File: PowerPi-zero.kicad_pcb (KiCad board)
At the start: 2 copper layers, 65 x 56 mm, 34 parts, among them J1 2444, J3 Conn_01x02, J6 Raspberry_Pi_2_3, J8 2444, Q1 30V 4A 44mΩ, Q2 50nA 150V 200mW 200mA, Q3 30V 4A 44mΩ, U1 XL4015

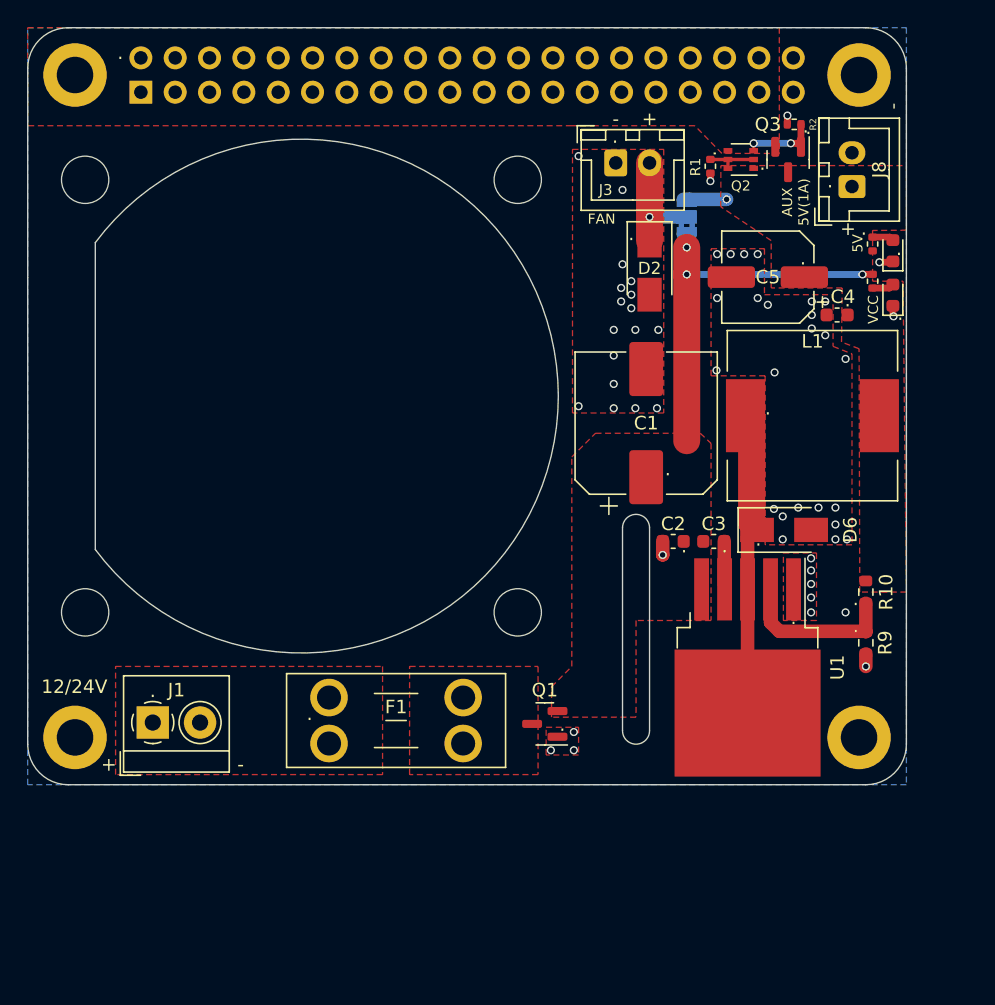
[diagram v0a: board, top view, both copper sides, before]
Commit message: Layout complete for PowerPi zero
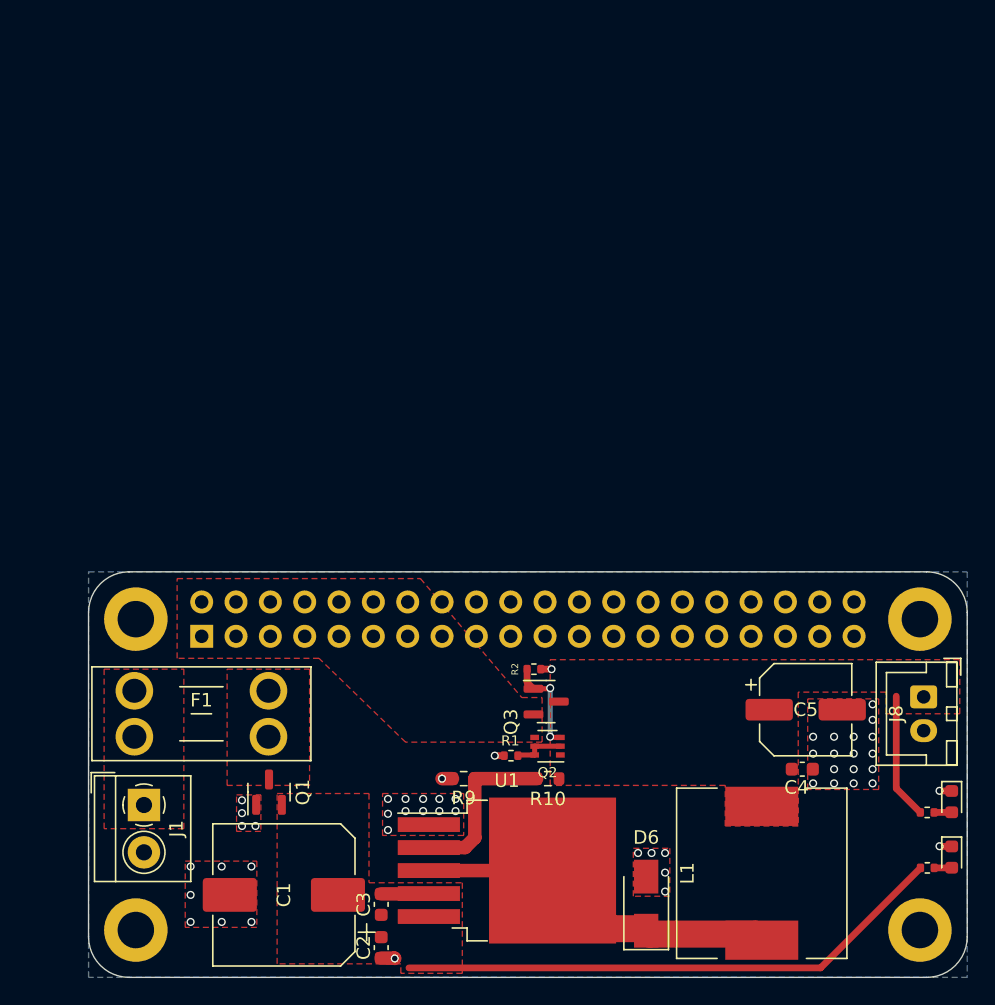
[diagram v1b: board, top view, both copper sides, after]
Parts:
- removed D2: SS54, Diode_SMD:D_SMA
- removed H5, H6, H7, H8: MountingHole, MountingHole:MountingHole_3.5mm
- removed J3: Conn_01x02, Connector_JST:JST_XH_B2B-XH-A_1x02_P2.50mm_Vertical
- removed JP1: SolderJumper_3_Bridged12, Jumper:SolderJumper-3_P1.3mm_Bridged2Bar12_RoundedPad1.0x1.5mm
- moved R1 46.0 mm to (121.0, 107.1), turned to 180 degrees
- moved Q2 45.7 mm to (123.7, 106.4)
- moved R2 44.7 mm to (122.7, 100.7), turned to 0 degrees
- moved C1 44.0 mm to (104.2, 117.4), turned to 180 degrees
- moved Q3 43.9 mm to (123.6, 103.1), turned to 0 degrees
- moved R8 43.6 mm to (151.8, 115.4), turned to 180 degrees
- moved R6 42.2 mm to (151.8, 111.3), turned to 180 degrees
- moved D5 41.8 mm to (153.6, 114.6), turned to -90 degrees
- moved D3 41.0 mm to (153.6, 110.5), turned to -90 degrees
- moved H2 40.5 mm to (93.2, 97.0)
- moved H3 40.5 mm to (151.2, 97.0)
- moved J6 40.5 mm to (98.1, 98.3)
- moved J8 38.1 mm to (151.5, 102.8), turned to -90 degrees
- moved C2 37.0 mm to (111.4, 121.3), turned to -90 degrees
- moved C3 36.4 mm to (111.4, 118.1), turned to -90 degrees
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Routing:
- net VCC: track 29.0 -> 40.9 mm, vias 3 -> 0
- net Net-(D2-Pad1): track 8.10 -> 0.00 mm, vias 1 -> 0
- net +5V: track 2.95 -> 9.34 mm, vias 1 -> 0
- net Net-(D6-Pad1): track 22.4 -> 26.8 mm
- net Net-(Q2-Pad3): track 5.83 -> 7.27 mm
- net Net-(R10-Pad1): track 12.0 -> 12.7 mm
- net GND: track 4.99 -> 5.08 mm, vias 56 -> 50
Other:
- board size 65 x 56 mm -> 65 x 30 mm
- board text added: "Select one of these board edges depending upon the type of socket that is used."
- board text removed: "+"
- board text removed: "-"
- board text removed: "."
- board text removed: "12/24V"
- board text removed: "5V"
- board text removed: "AUX 5V(1A)"
- board text removed: "FAN"
- board text removed: "JLCJLCJLC"
- board text removed: "VCC"
- board text removed: "Vector 3D PowerPi Designed by Sreenivas Eadara"

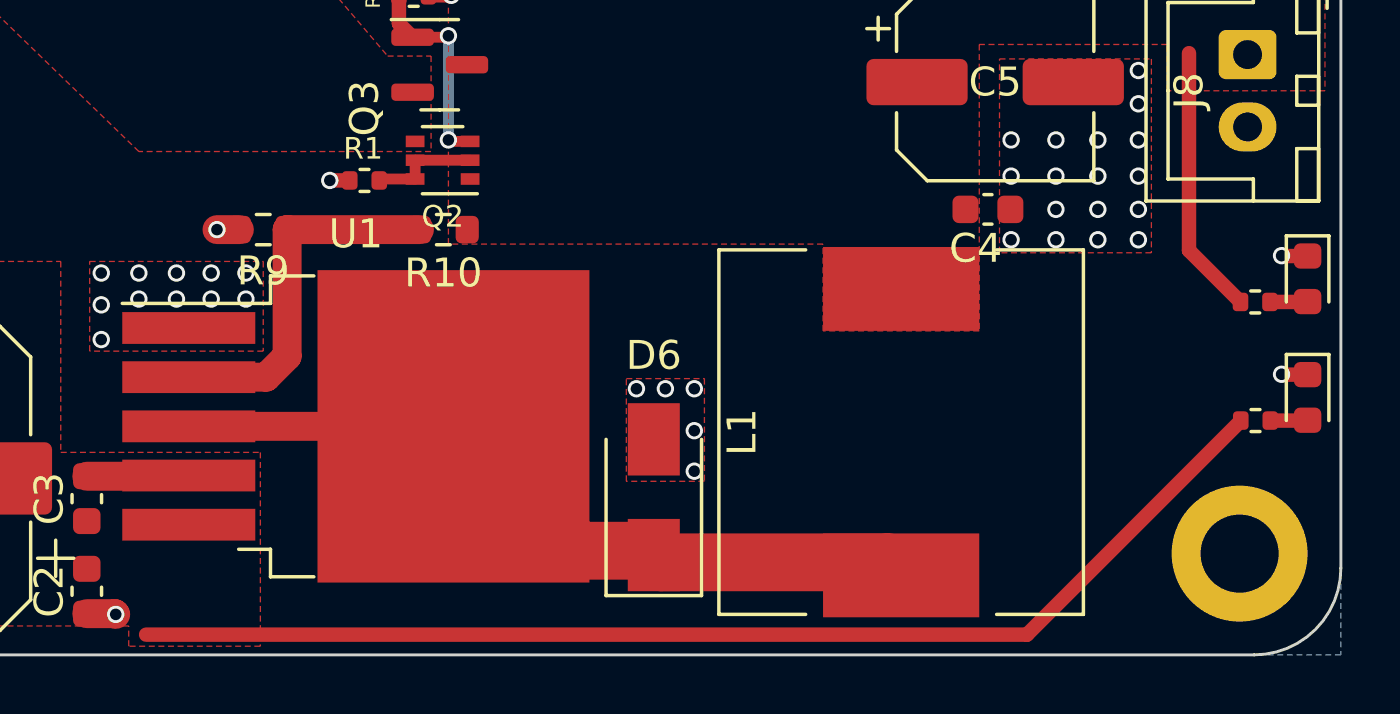
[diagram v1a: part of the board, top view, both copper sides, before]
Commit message: cleanup
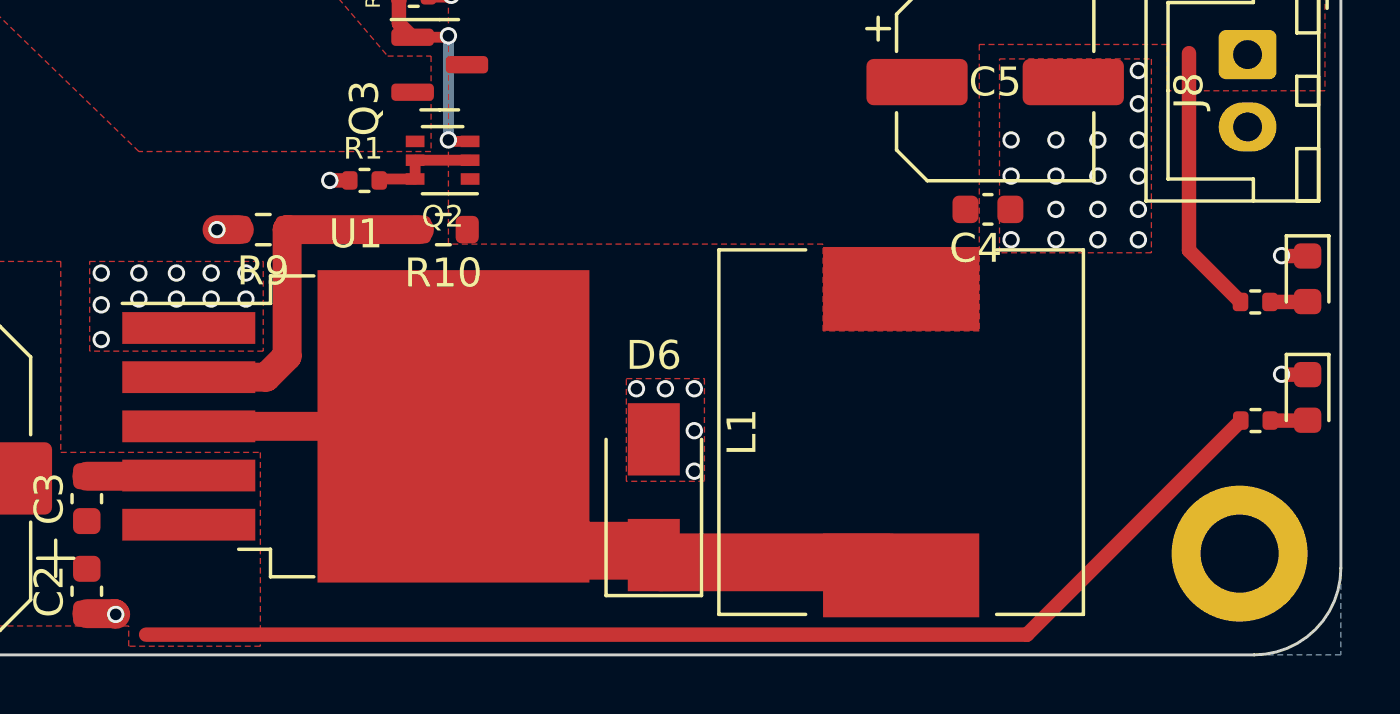
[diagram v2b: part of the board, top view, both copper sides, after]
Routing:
- net Net-(D6-Pad1): track 26.8 -> 26.1 mm
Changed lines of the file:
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@@
     (style (thickness 0.15) (arrow_length 1.27) (text_position_mode 0) (extension_height 0.58642) (extension_offset 0) keep_text_aligned)
   )
-  (segment (start 151.29 115.4) (end 151.29 115.41) (width 0.5) (layer "F.Cu") (net 1))
   (segment (start 151.29 115.41) (end 143.9 122.8) (width 0.5) (layer "F.Cu") (net 1))
   (segment (start 143.9 122.8) (end 113.45 122.8) (width 0.5) (layer "F.Cu") (net 1))
@@
   (via (at 119.8 107.1) (size 0.6) (drill 0.4) (layers "F.Cu" "B.Cu") (net 2))
   (segment (start 111.4 117.325) (end 114.9 117.325) (width 1) (layer "F.Cu") (net 3))
-  (segment (start 114.9 117.325) (end 114.925 117.3) (width 1) (layer "F.Cu") (net 3))
   (segment (start 151.280001 111.3) (end 149.5 109.519999) (width 0.5) (layer "F.Cu") (net 4))
   (segment (start 149.5 109.519999) (end 149.5 102.7) (width 0.5) (layer "F.Cu") (net 4))
-  (segment (start 153.5875 111.3) (end 153.6 111.2875) (width 0.5) (layer "F.Cu") (net 5))
   (segment (start 152.300001 111.3) (end 153.5875 111.3) (width 0.5) (layer "F.Cu") (net 5))
-  (segment (start 153.5875 115.4) (end 153.6 115.3875) (width 0.5) (layer "F.Cu") (net 6))
   (segment (start 152.31 115.4) (end 153.5875 115.4) (width 0.5) (layer "F.Cu") (net 6))
-  (segment (start 139.55 120.75) (end 139.1 120.3) (width 2) (layer "F.Cu") (net 7))
   (segment (start 128.375 119.9) (end 124.075 115.6) (width 2) (layer "F.Cu") (net 7))
   (segment (start 131.25 120.3) (end 131 120.05) (width 2) (layer "F.Cu") (net 7))
@@
   (segment (start 139.1 120.3) (end 131.25 120.3) (width 2) (layer "F.Cu") (net 7))
   (segment (start 122.75 107.05) (end 121.56 107.05) (width 0.375) (layer "F.Cu") (net 31))
-  (segment (start 121.56 107.05) (end 121.51 107.1) (width 0.375) (layer "F.Cu") (net 31))
   (segment (start 122.75 106.4) (end 124.65 106.4) (width 0.375) (layer "F.Cu") (net 31))
   (segment (start 122.75 107.05) (end 122.75 106.4) (width 0.375) (layer "F.Cu") (net 31))
